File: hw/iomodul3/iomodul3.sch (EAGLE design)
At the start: 56 parts, among them IC1 MCP2551, IC3 STM32F042K, IC4 MCP1700T3302E/TT, IC5 DS8289, Q2 8MHz

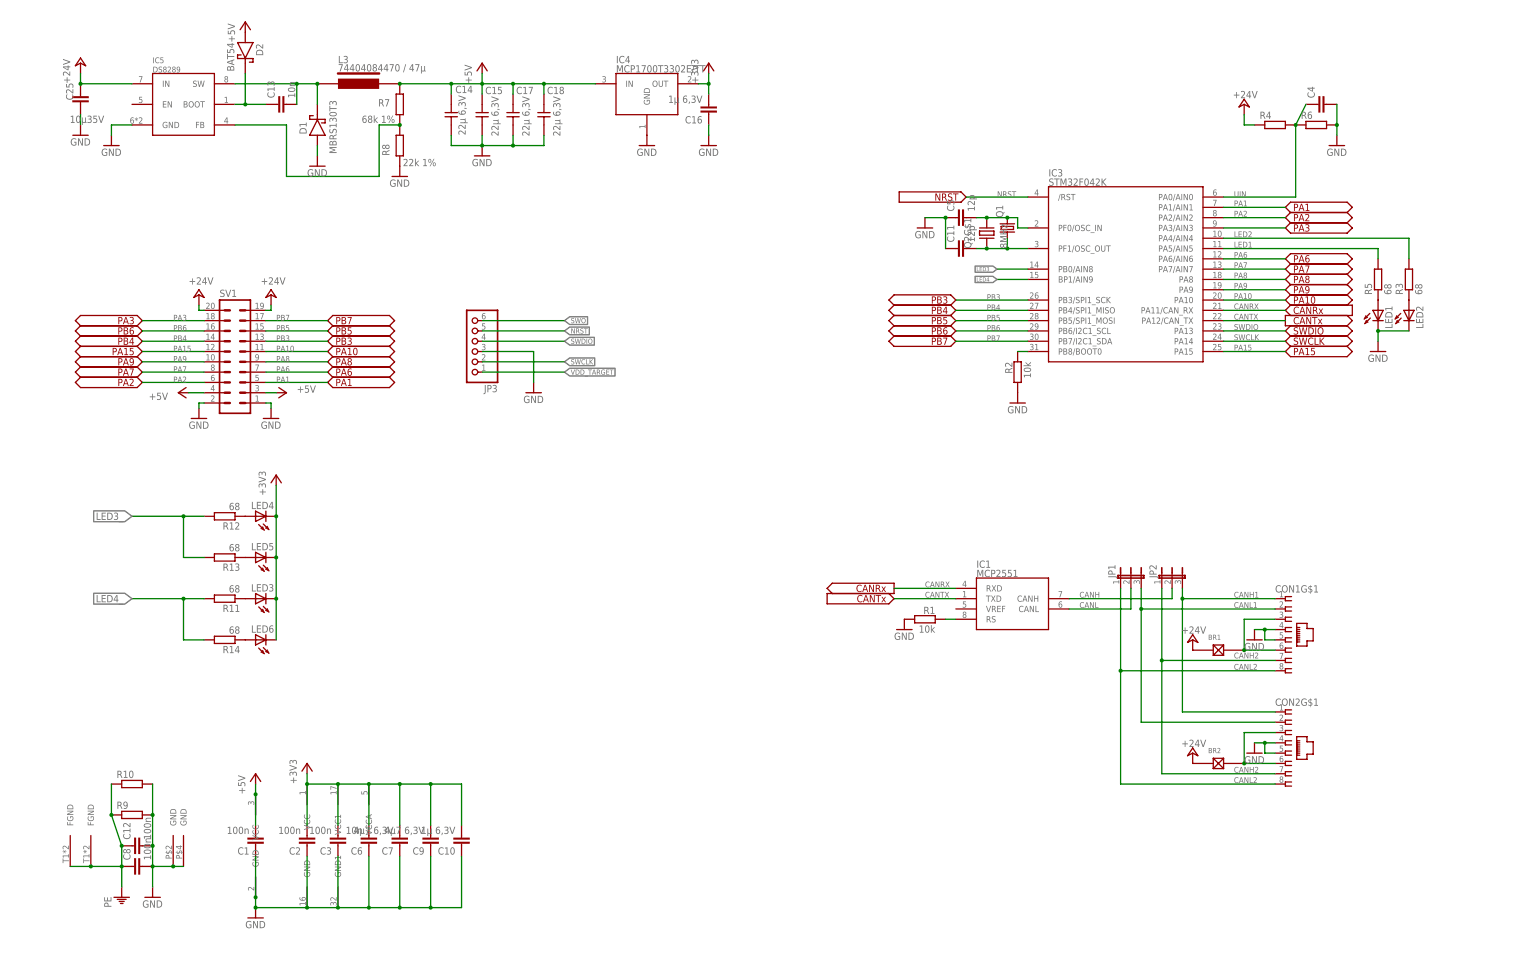
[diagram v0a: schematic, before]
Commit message: board version 3 begonnen
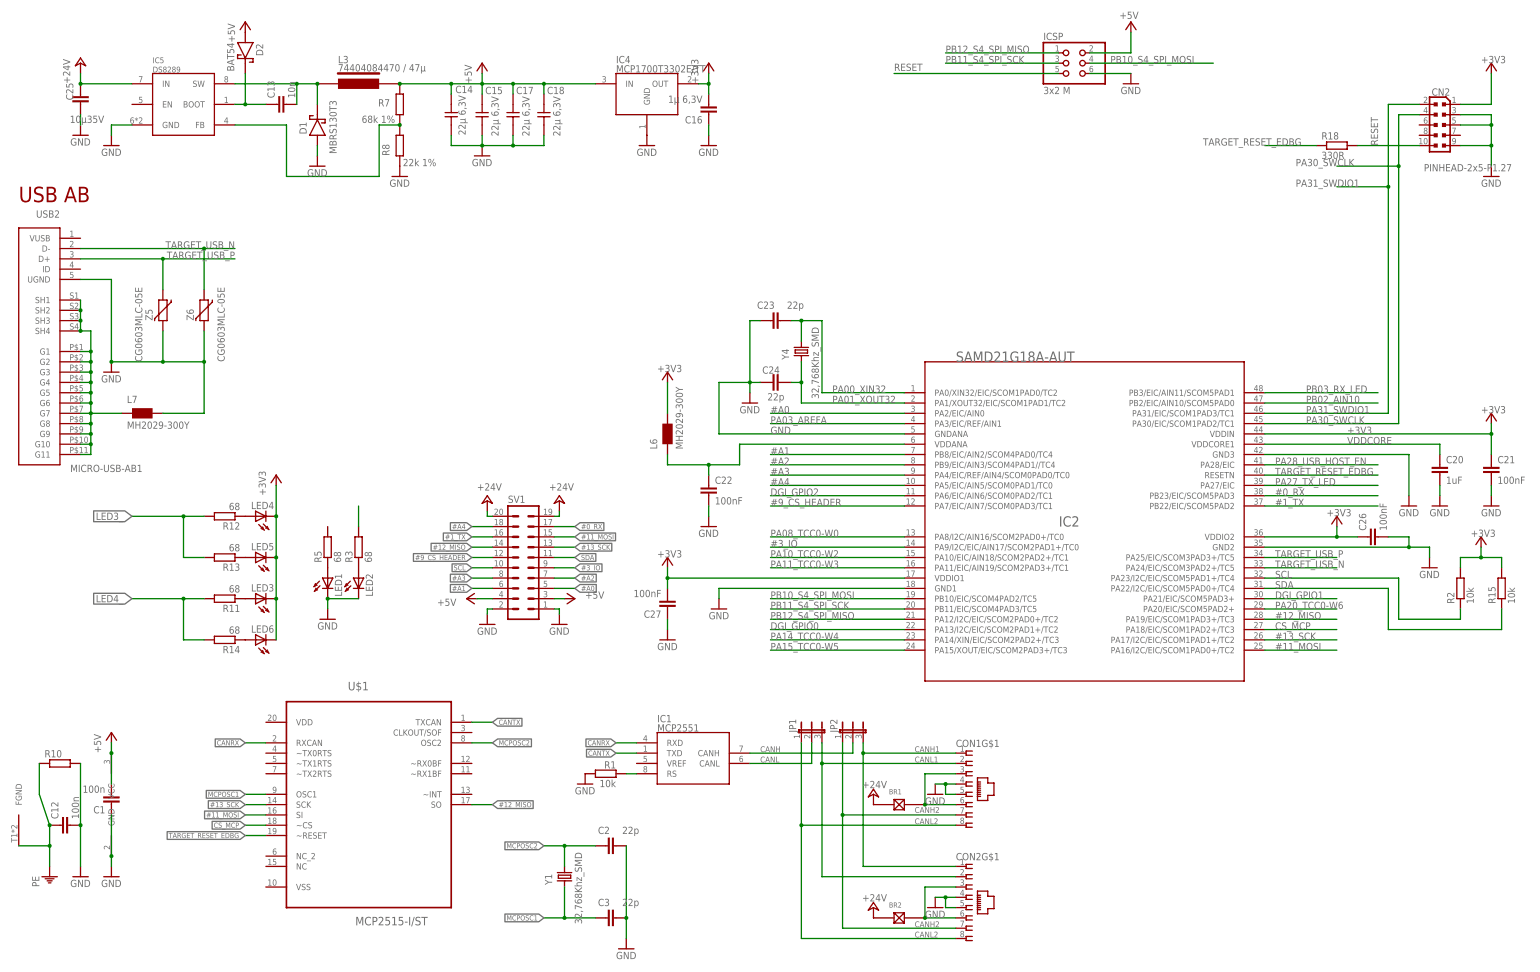
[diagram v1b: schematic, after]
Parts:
- removed C10: 1µ 6,3V, schlager_passiv:C-EUC0805
- removed C11, C5: 12p, schlager_passiv:C-EUC0805
- removed C4: (no value), schlager_passiv:C-EUC0805
- removed C6: 10n, schlager_passiv:C-EUC0805
- removed C7, C9: 4µ7 6,3V, schlager_passiv:C-EUC0805
- removed C8: 100n, schlager_passiv:C-EUC0805
- removed IC3: STM32F042K, MYSGS:STM32F042
- removed JP3: (no value), pinhead:PINHD-1X6
- removed Q1: (no value), crystal:CRYSTALHC49U-V
- removed Q2: 8MHz, MYPASS:MT-CRYSTAL
- removed R4, R6, R9: (no value), schlager_passiv:R-EU_R0805
- added C20: 1uF, schlager_passiv:C-EUC0805
- added C21, C22, C26, C27: 100nF, schlager_passiv:C-EUC0805
- added C23, C24: 22p, schlager_passiv:C-EUC0805
- added CN2: PINHEAD-2x5-P1.27, Connettori:0171_PH127-205DF055G00A
- added IC2: SAMD21G18A-AUT, IntegratedCircuits:1792_SAMD21G18A-AUT
- added ICSP: 3x2 M, Connettori:0114_PH254-203DF118A00V
- added L6, L7: MH2029-300Y, Protezione:0001_BLM21PG300SN1D_/_MH2029-300Y
- added R15: 10k, schlager_passiv:R-EU_R0805
- added R18: 330R, schlager_passiv:R-EU_R0805
- added U$1: MCP2515-I/ST, CHIP_MCP:MCP2515-I/ST
- added USB2: MICRO-USB-AB1, Connettori:0631_MCR-AB1-S-RA-SMT-TR
- added Y1, Y4: 32,768Khz_SMD, Cristalli:0213_ABS07-32.768KHZ-T
- added Z5, Z6: CG0603MLC-05E, Protezione:0010_BRNCG0603MLC-05E
- C2, C3: value 100n -> 22p
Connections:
- removed net LED1: IC3G$1.PA5/AIN5, R5.2
- removed net N$5: C5.2, IC3G$1.PF0/OSC_IN, Q1.2, Q2G$1.2
- removed net NRST: IC3G$1./RST, JP3.5
- removed net PA1: IC3G$1.PA1/AIN1, SV1.5
- removed net PA10: IC3G$1.PA10, SV1.11
- removed net PA15: IC3G$1.PA15, SV1.12
- removed net PA2: IC3G$1.PA2/AIN2, SV1.6
- removed net PA3: IC3G$1.PA3/AIN3, SV1.18
- removed net PA6: IC3G$1.PA6/AIN6, SV1.7
- removed net PA7: IC3G$1.PA7/AIN7, SV1.8
- removed net PA8: IC3G$1.PA8, SV1.9
- removed net PA9: IC3G$1.PA9, SV1.10
- removed net PB3: IC3G$1.PB3/SPI1_SCK, SV1.13
- removed net PB4: IC3G$1.PB4/SPI1_MISO, SV1.14
- removed net PB5: IC3G$1.PB5/SPI1_MOSI, SV1.15
- removed net PB6: IC3G$1.PB6/I2C1_SCL, SV1.16
- removed net PB7: IC3G$1.PB7/I2C1_SDA, SV1.17
- removed net SWCLK: IC3G$1.PA14, JP3.2
- removed net SWDIO: IC3G$1.PA13, JP3.4
- removed net SWO: JP3.6
- removed net UIN: C4.1, IC3G$1.PA0/AIN0, R4.2, R6.1
- removed net VDD_TARGET: JP3.1
- new net #0_RX: IC2.PB23/EIC/SCOM5PAD3, SV1.17
- new net #11_MOSI: IC2.PA16/I2C/EIC/SCOM1PAD0+/TC2, SV1.15, U$1.SI
- new net #12_MISO: IC2.PA19/EIC/SCOM1PAD3+/TC3, SV1.14, U$1.SO
- new net #13_SCK: IC2.PA17/I2C/EIC/SCOM1PAD1+/TC2, SV1.13, U$1.SCK
- new net #1_TX: IC2.PB22/EIC/SCOM5PAD2, SV1.16
- new net #3_IO: IC2.PA9/I2C/EIC/AIN17/SCOM2PAD1+/TC0, SV1.9
- new net #9_CS_HEADER: IC2.PA7/EIC/AIN7/SCOM0PAD3/TC1, SV1.12
- new net #A0: IC2.PA2/EIC/AIN0, SV1.5
- new net #A1: IC2.PB8/EIC/AIN2/SCOM4PAD0/TC4, SV1.6
- new net #A2: IC2.PB9/EIC/AIN3/SCOM4PAD1//TC4, SV1.7
- new net #A3: IC2.PA4/EIC/REF/AIN4/SCOM0PAD0/TC0, SV1.8
- new net #A4: IC2.PA5/EIC/AIN5/SCOM0PAD1/TC0, SV1.18
- new net CS_MCP: IC2.PA18/EIC/SCOM1PAD2+/TC3, U$1.~CS
- new net DGI_GPIO0: IC2.PA13/I2C/EIC/SCOM2PAD1+/TC2
- new net DGI_GPIO1: IC2.PA21/EIC/SCOM5PAD3+
- new net DGI_GPIO2: IC2.PA6/EIC/AIN6/SCOM0PAD2/TC1
- new net MCPOSC1: C3.1, U$1.OSC1, Y1.1
- new net MCPOSC2: C2.1, U$1.OSC2, Y1.2
- new net PA00_XIN32: C23.2, IC2.PA0/XIN32/EIC/SCOM1PAD0/TC2, Y4.2
- new net PA01_XOUT32: C24.2, IC2.PA1/XOUT32/EIC/SCOM1PAD1/TC2, Y4.1
- new net PA03_AREFA: IC2.PA3/EIC/REF/AIN1
- new net PA08_TCC0-W0: IC2.PA8/I2C/AIN16/SCOM2PAD0+/TC0
- new net PA10_TCC0-W2: IC2.PA10/EIC/AIN18/SCOM2PAD2+/TC1
- new net PA11_TCC0-W3: IC2.PA11/EIC/AIN19/SCOM2PAD3+/TC1
- new net PA14_TCC0-W4: IC2.PA14/XIN/EIC/SCOM2PAD2+/TC3
- new net PA15_TCC0-W5: IC2.PA15/XOUT/EIC/SCOM2PAD3+/TC3
- new net PA20_TCC0-W6: IC2.PA20/EIC/SCOM5PAD2+
- new net PA27_TX_LED: IC2.PA27/EIC
- new net PA28_USB_HOST_EN: IC2.PA28/EIC
- new net PA30_SWCLK: CN2.4, IC2.PA30/EIC/SCOM1PAD2/TC1
- new net PA31_SWDIO1: CN2.2, IC2.PA31/EIC/SCOM1PAD3/TC1
- new net PB02_AIN10: IC2.PB2/EIC/AIN10/SCOM5PAD0
- new net PB03_RX_LED: IC2.PB3/EIC/AIN11/SCOM5PAD1
- new net PB10_S4_SPI_MOSI: IC2.PB10/EIC/SCOM4PAD2/TC5, ICSP.4
- new net PB11_S4_SPI_SCK: IC2.PB11/EIC/SCOM4PAD3/TC5, ICSP.3
- new net PB12_S4_SPI_MISO: IC2.PA12/I2C/EIC/SCOM2PAD0+/TC2, ICSP.1
- new net RESET: CN2.10, ICSP.5, R18.2
- new net SCL: IC2.PA23/I2C/EIC/SCOM5PAD1+/TC4, R2.1, SV1.10
- new net SDA: IC2.PA22/I2C/EIC/SCOM5PAD0+/TC4, R15.1, SV1.11
- new net TARGET_RESET_EDBG: IC2.RESETN, R18.1, U$1.~RESET
- new net TARGET_USB_N: IC2.PA24/EIC/SCOM3PAD2+/TC5, USB2.D-, Z6.1
- new net TARGET_USB_P: IC2.PA25/EIC/SCOM3PAD3+/TC5, USB2.D+, Z5.1
- new net VDDCORE: C20.1, IC2.VDDCORE1
- net +24V: no longer R4.1
- net +3V3: now also C21.1, C26.1, C27.2, CN2.1, IC2.VDDIN, IC2.VDDIO1, IC2.VDDIO2, L6.2, R15.2, R2.2; no longer C10.2, C2.2, C3.2, C6.2, C7.2, C9.2, IC3G$2.VCC, IC3G$2.VCC1, IC3G$2.VCCA
- net +5V: now also ICSP.2
- net CANRX: now also U$1.RXCAN; no longer IC3G$1.PA11/CAN_RX
- net CANTX: now also U$1.TXCAN; no longer IC3G$1.PA12/CAN_TX
- net GND: now also C2.2, C20.2, C21.2, C22.2, C23.1, C24.1, C26.2, C27.1, C3.2, CN2.3, CN2.5, CN2.9, IC2.GND1, IC2.GND2, IC2.GND3, IC2.GNDANA, ICSP.6, L7.2, USB2.UGND, Z5.2, Z6.2; no longer C10.1, C11.1, C2.1, C3.1, C4.2, C5.1, C6.1, C7.1, C8.2, C9.1, IC3G$2.GND, IC3G$2.GND1, JP3.3, Q2G$2.GND, Q2G$3.GND, R2.2, R6.2, R9.2
- net LED2: no longer IC3G$1.PA4/AIN4
- net LED3_: no longer IC3G$1.PB0/AIN8
- net LED4_: no longer IC3G$1.BP1/AIN9
- net N$15: now also C22.1, IC2.VDDANA, L6.1; no longer IC3G$1.PB8/BOOT0, R2.1
- net N$4: now also L7.1, USB2.G1, USB2.G10, USB2.G11, USB2.G2, USB2.G3, USB2.G4, USB2.G5, USB2.G6, USB2.G7, USB2.G8, USB2.G9, USB2.SH1, USB2.SH2, USB2.SH3, USB2.SH4; no longer C11.2, IC3G$1.PF1/OSC_OUT, Q1.1, Q2G$1.1
- net PE: no longer C8.1, CON2G$2.FGND, R9.1
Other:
- note added: "USB AB"
- moved on the sheet: BR1, BR2, C1, C12, C2, C3, CON1G$1, CON2G$1, IC1, JP1, JP2, LED1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
